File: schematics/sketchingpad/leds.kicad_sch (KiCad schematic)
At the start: 25 parts

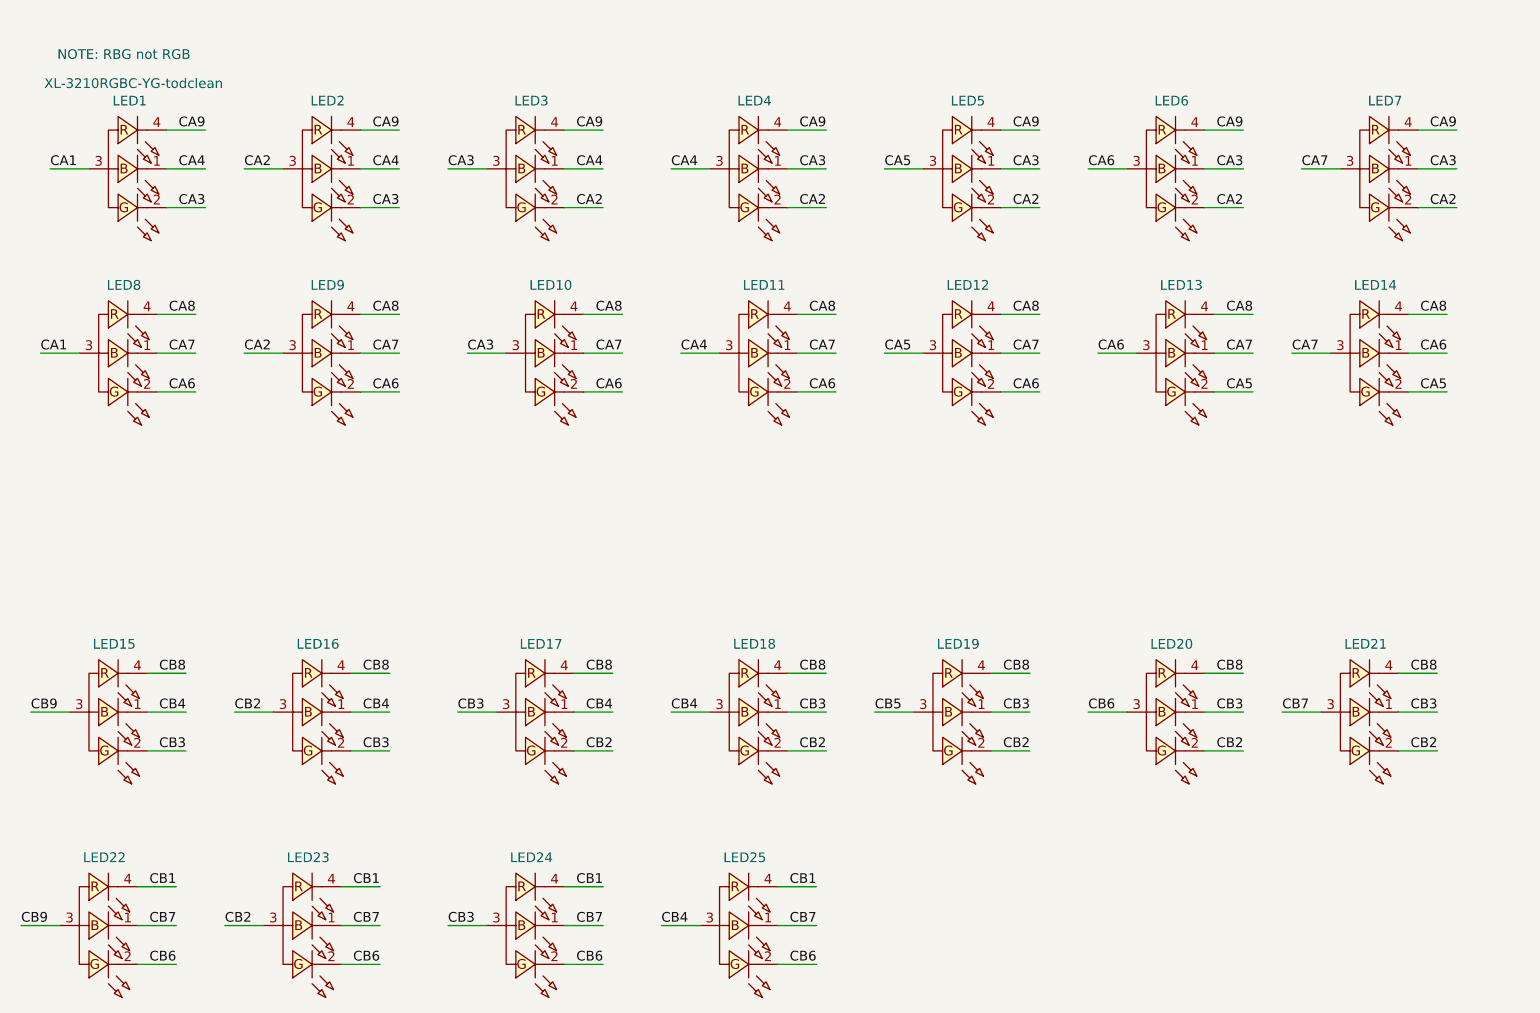
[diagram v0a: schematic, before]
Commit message: some pcb layout for touch
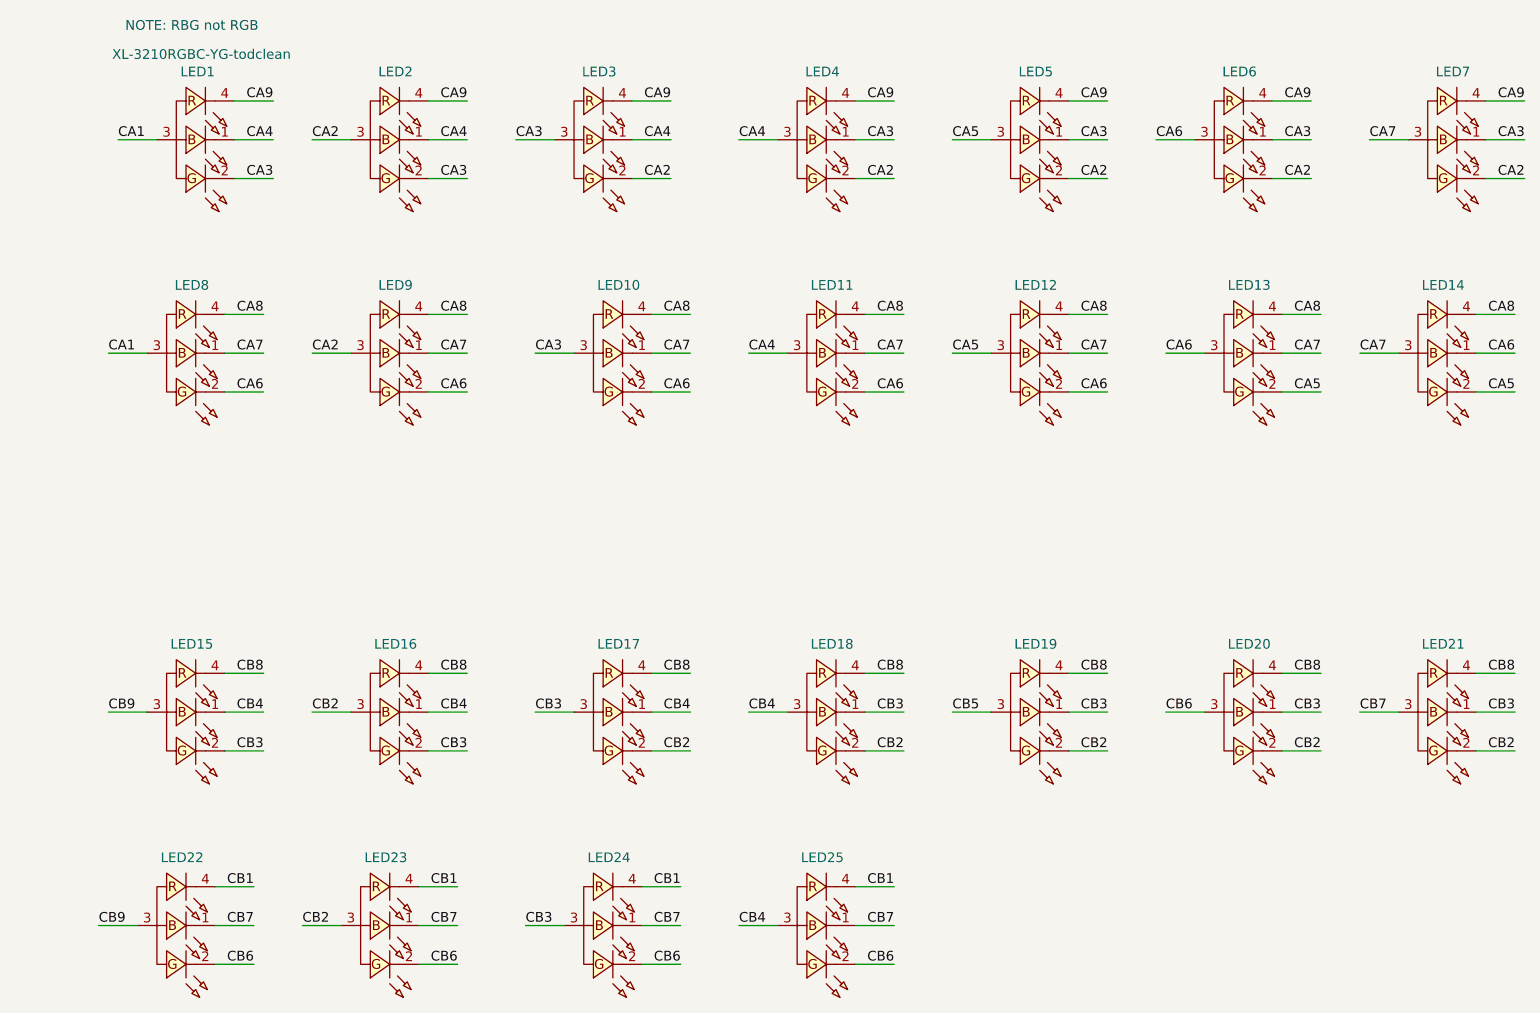
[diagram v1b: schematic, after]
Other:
- moved on the sheet: LED1, LED10, LED11, LED12, LED13, LED14, LED15, LED16, LED17, LED18, LED19, LED2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
